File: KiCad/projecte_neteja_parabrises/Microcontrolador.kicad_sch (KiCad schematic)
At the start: 11 parts, among them J1 Conn_01x09_Pin, U1 PIC24HJ32GP302, U2 SN74LVC2T45DCUR, U3 HDC2080, Y1 Crystal

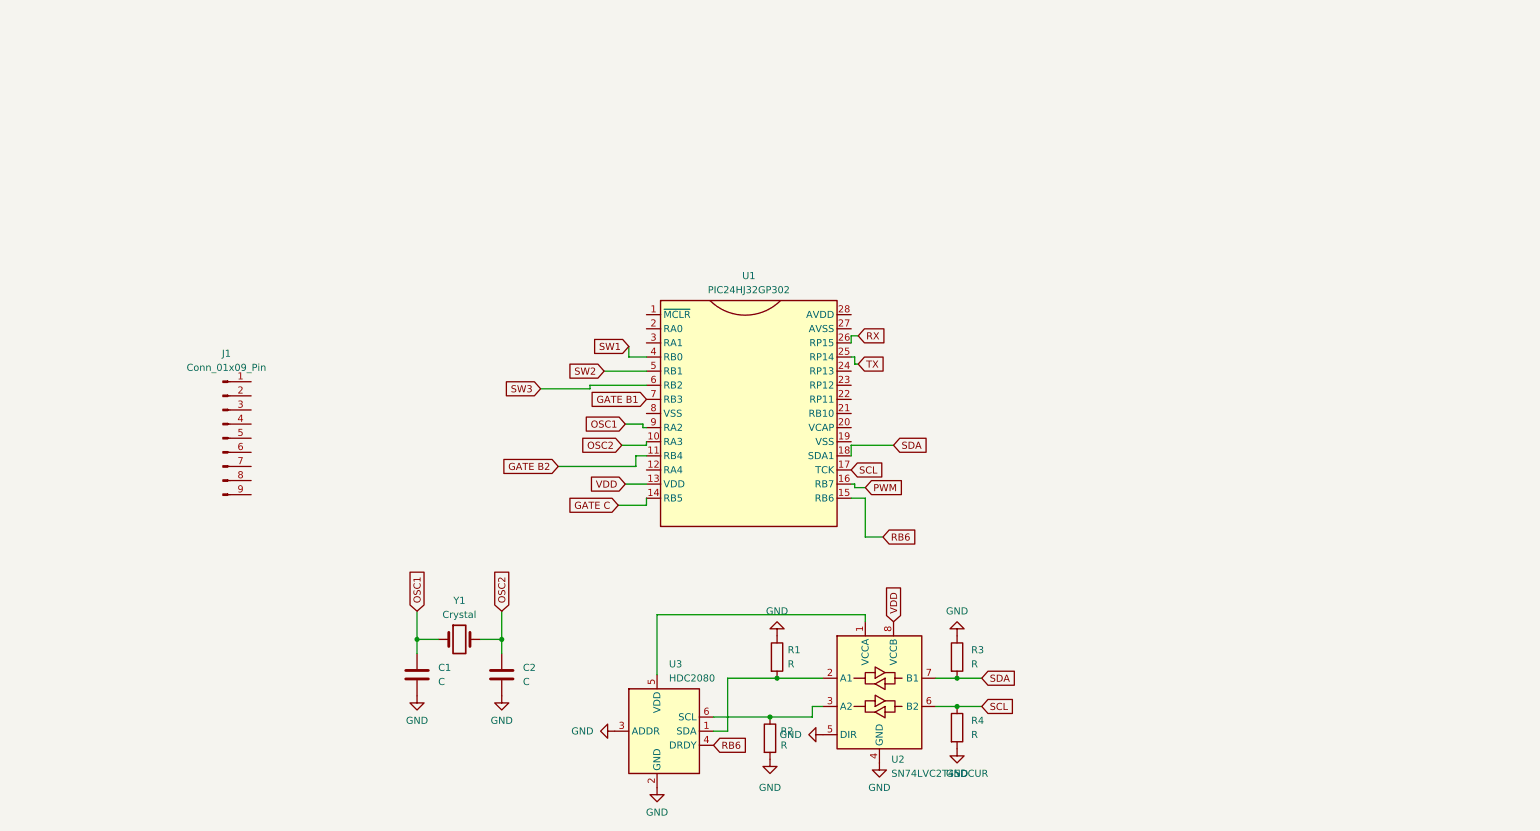
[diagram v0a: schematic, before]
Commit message: SCH V1
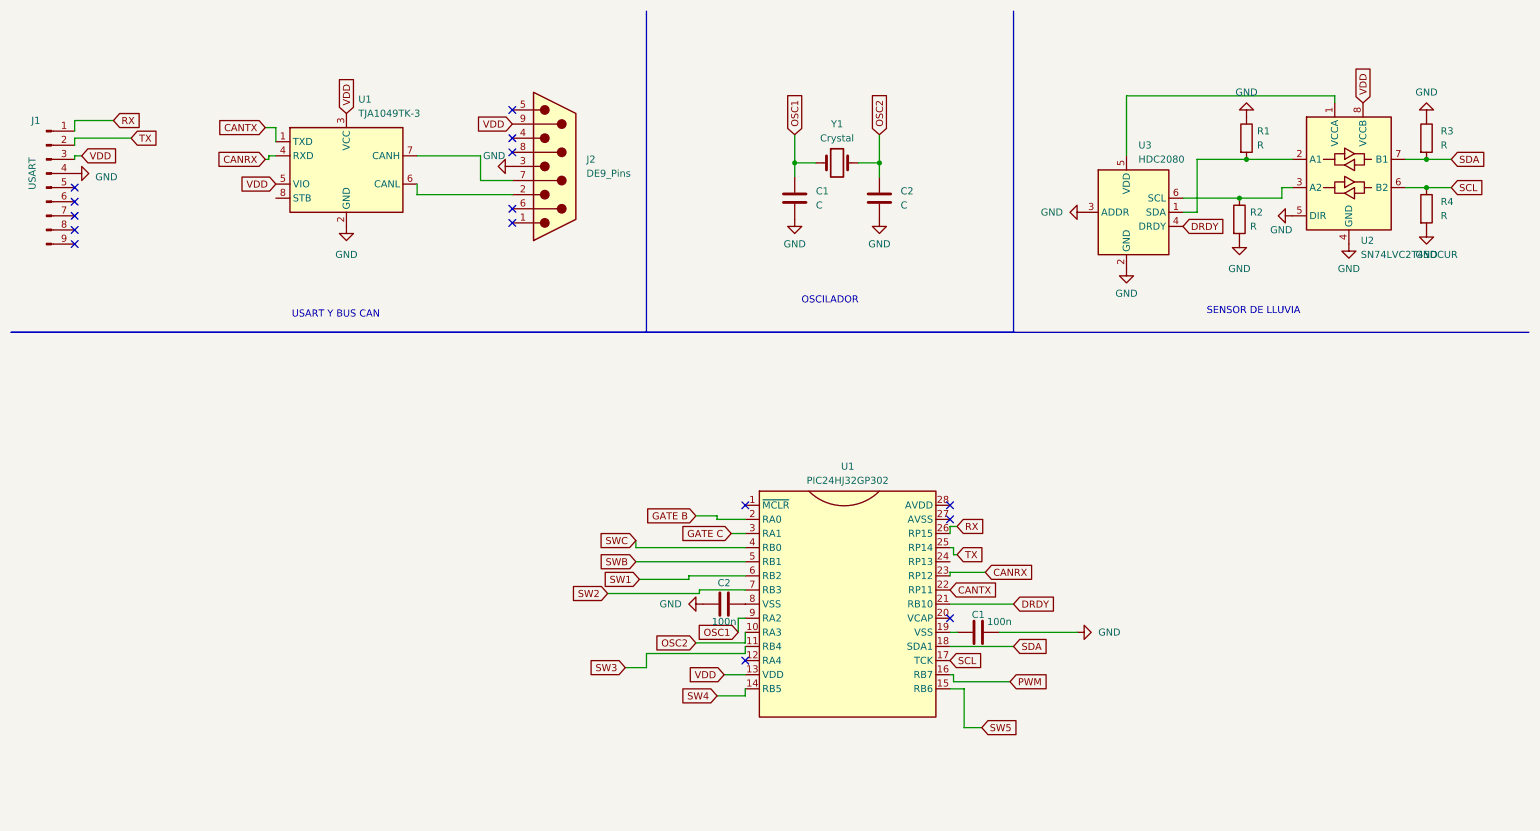
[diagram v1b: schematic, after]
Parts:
- added C1, C2: 100n, symbol Device:C
- added J2: DE9_Pins, symbol Connector:DE9_Pins
- added U1: TJA1049TK-3, Package_SON:HVSON-8-1EP_3x3mm_P0.65mm_EP1.6x2.4mm, symbol Interface_CAN_LIN:TJA1049TK-3
- J1: value Conn_01x09_Pin -> USART
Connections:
- net GATE B1 is gone; now on net SW2: U1.7 (RB3)
- net GATE B2 is gone; now on net SW3: U1.11 (RB4)
- net GATE C: now also U1.3 (RA1); no longer U1.14 (RB5)
- net GND: now also J1.4 (Pin_4), C1.2, C2.1, J2.3, U1.2 (GND), U1.9 (GND)
- net RX: now also J1.1 (Pin_1)
- net SW1: now also U1.6 (RB2); no longer U1.4 (RB0)
- net SW2: no longer U1.5 (RB1)
- net SW3: no longer U1.6 (RB2)
- net TX: now also J1.2 (Pin_2)
- net VDD: now also J1.3 (Pin_3), J2.9, U1.3 (VCC), U1.5 (VIO)
- net at U1.19 (VSS): now also C1.1
- net GATE B: now reaches U1.2 (RA0)
- net DRDY: now reaches U1.21 (RB10)
- net DRDY: now also U3.4 (DRDY)
- net CANTX: now reaches U1.22 (RP11)
- net CANTX: now also U1.1 (TXD)
- net CANRX: now reaches U1.23 (RP12)
- net CANRX: now also U1.4 (RXD)
- net at U1.8 (VSS): now also C2.2
- net RB6 renamed SW5
- net SW5: no longer U3.4 (DRDY)
- new net: J2.2, U1.6 (CANL)
- new net: J2.7, U1.7 (CANH)
- new net SW4: U1.14 (RB5)
- new net SWB: U1.5 (RB1)
- new net SWC: U1.4 (RB0)
- no-connect marks 0 -> 15
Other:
- note added: "OSCILADOR"
- note added: "SENSOR DE LLUVIA"
- note added: "USART Y BUS CAN"
- moved on the sheet: C1, C2, J1, R1, R2, R3, R4, U1, U2, U3, Y1
